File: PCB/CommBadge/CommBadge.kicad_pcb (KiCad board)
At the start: 2 copper layers, 49.3 x 39.8 mm, 46 parts, among them J1 Reset, J2 Battery, J3 TC2030-USB-NL-DS, J5 USB-C-Socket-H, Q1 CJ2301, SW2 SW_Push, U2 MAX98357A, U3 TP4054, U4 ME6211C33M5G-N, U5 L, U6 ESP32-S3-MINI-1, U7 R

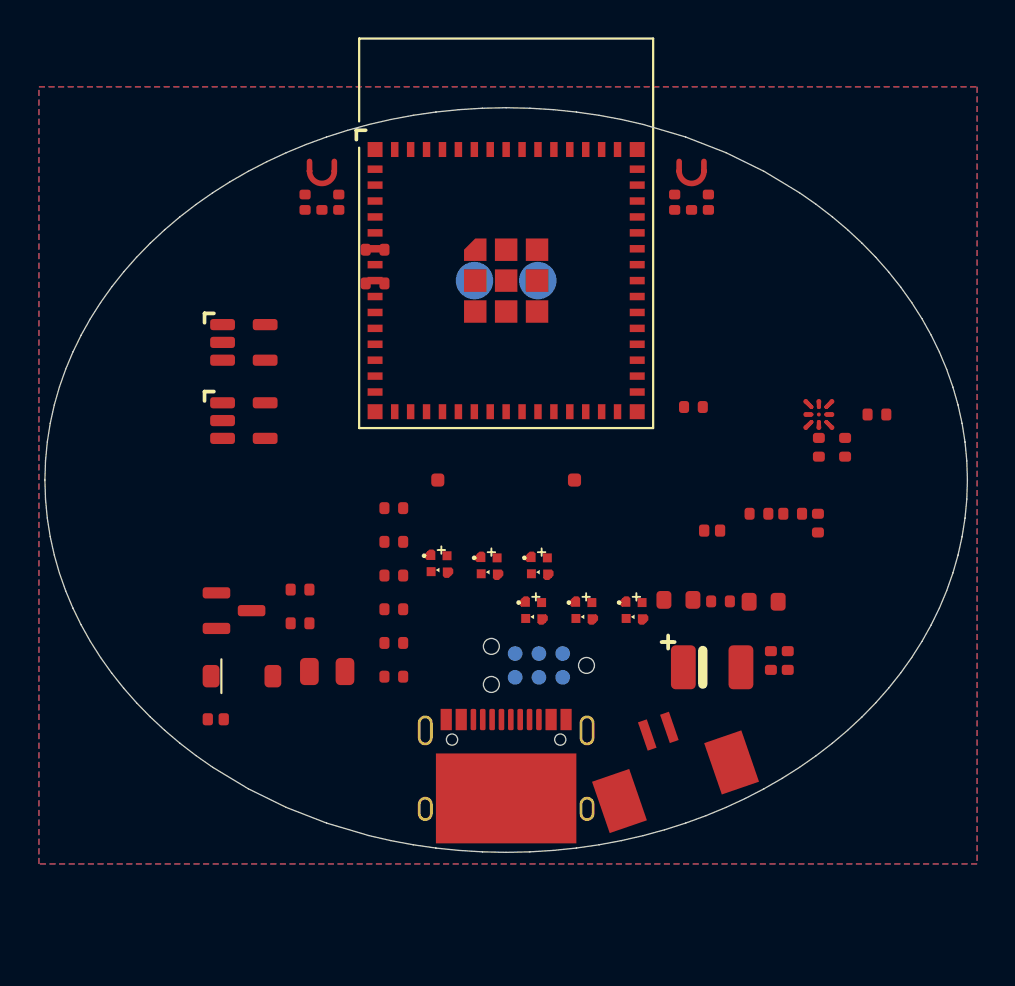
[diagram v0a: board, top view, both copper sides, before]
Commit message: Components
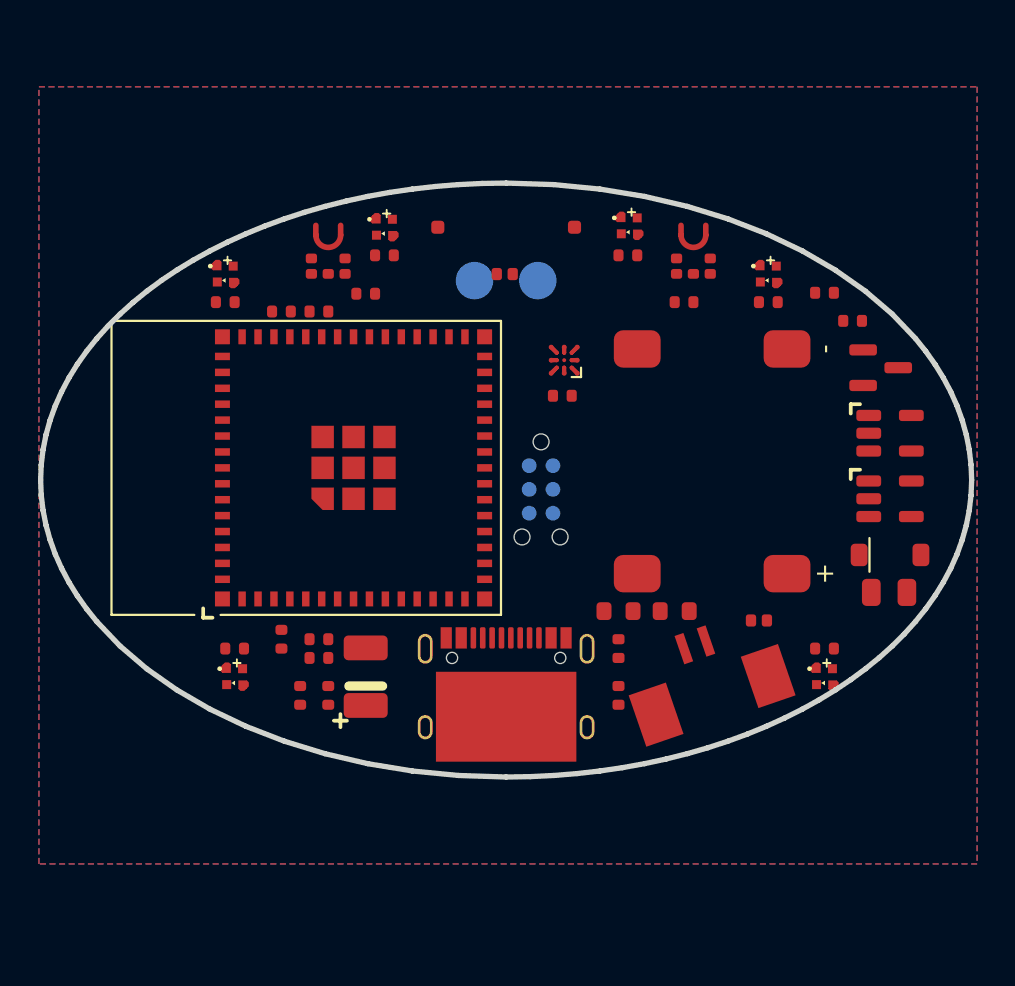
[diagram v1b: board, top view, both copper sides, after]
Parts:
- added LS1: Speaker, RevK:KLJ-Speaker, F.Cu at (111.0, 94.5)
- moved Q1 36.9 mm to (120.0, 89.5)
- moved D2 35.2 mm to (120.5, 99.5)
- moved U3 34.8 mm to (120.5, 93.0)
- moved U4 34.8 mm to (120.5, 96.5)
- moved R3 33.6 mm to (118.5, 87.0)
- moved R1 32.2 mm to (117.0, 85.5)
- moved C13 30.7 mm to (89.0, 107.0)
- moved C14 30.6 mm to (90.5, 107.0)
- moved C4 30.3 mm to (120.5, 101.5)
- moved D1 29.5 mm to (113.5, 103.0)
- moved C7 29.3 mm to (88.0, 104.0)
- moved D7 28.3 mm to (85.0, 84.5)
- moved C9 27.7 mm to (88.0, 86.5)
- moved R2 27.5 mm to (90.0, 86.5)
- moved C15 24.8 mm to (114.0, 86.0)
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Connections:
- C11 pad 1: Net-(D4-+) -> +3V3
- C11 pad 2: Net-(D4--) -> GND
- C12 pad 1: Net-(D4-+) -> +3V3
- C12 pad 2: Net-(D4--) -> GND
- C15 pad 1: Net-(D4-+) -> +3V3
- C15 pad 2: Net-(D4--) -> GND
- C16 pad 1: Net-(D4-+) -> +3V3
- C16 pad 2: Net-(D4--) -> GND
- C17 pad 1: Net-(D4-+) -> +3V3
- C17 pad 2: Net-(D4--) -> GND
- C18 pad 1: Net-(D4-+) -> +3V3
- C18 pad 2: Net-(D4--) -> GND
- C5 pad 1: DC -> VBUS
- D4 pad 2: Net-(D4-+) -> +3V3
- D4 pad 3: Net-(D4--) -> GND
- D5 pad 2: Net-(D4-+) -> +3V3
- D5 pad 3: Net-(D4--) -> GND
- D6 pad 2: Net-(D4-+) -> +3V3
- D6 pad 3: Net-(D4--) -> GND
- D7 pad 2: Net-(D4-+) -> +3V3
- D7 pad 3: Net-(D4--) -> GND
- D8 pad 2: Net-(D4-+) -> +3V3
- D8 pad 3: Net-(D4--) -> GND
- D9 pad 2: Net-(D4-+) -> +3V3
- D9 pad 3: Net-(D4--) -> GND
- J3 pad 1: DC -> VBUS
- J3 pad 2: DC -> VBUS
- J5 pad A4: DC -> VBUS
- J5 pad A9: DC -> VBUS
- J5 pad B4: DC -> VBUS
- J5 pad B9: DC -> VBUS
- U2 pad A3: unconnected-(U2-OUTP-PadA3) -> Net-(U2-OUTP)
- U2 pad B3: unconnected-(U2-OUTN-PadB3) -> Net-(U2-OUTN)
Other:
- board size 49.3 x 39.8 mm -> 49.7 x 31.7 mm

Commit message: Tweak
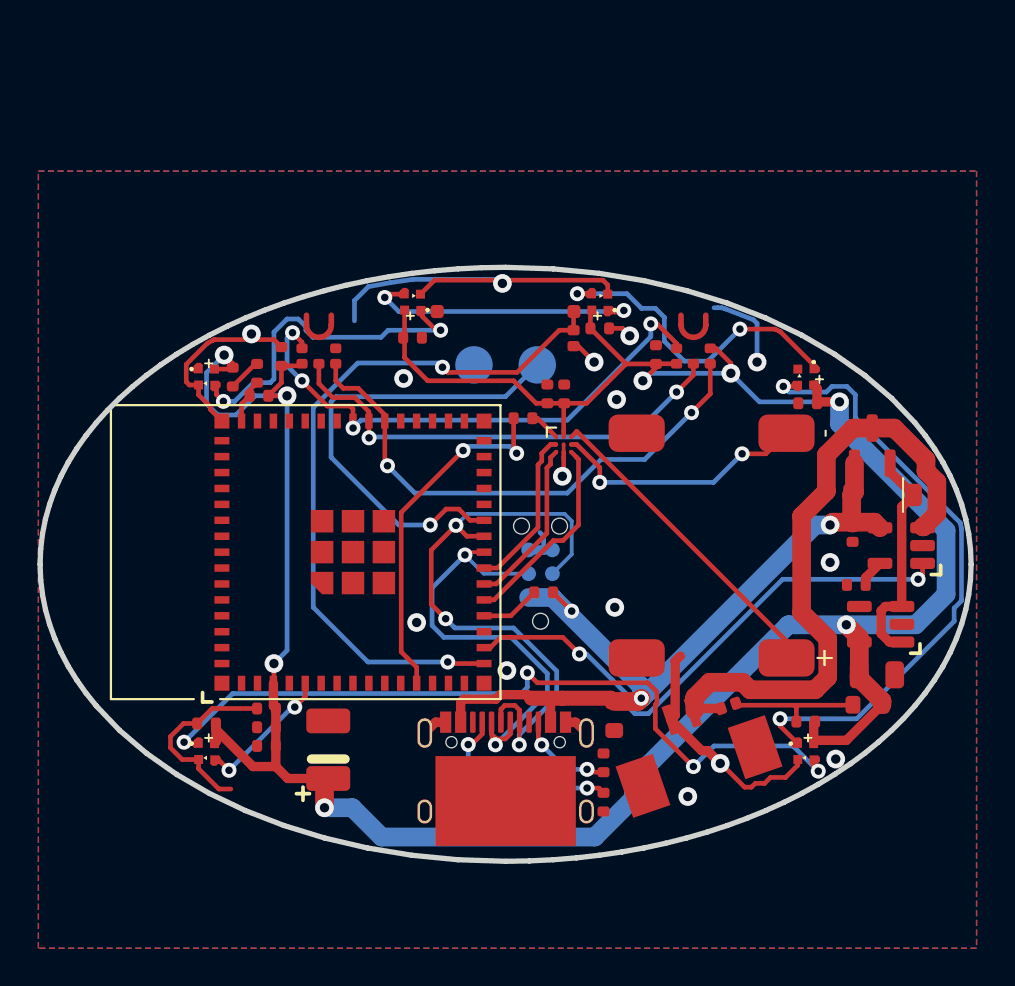
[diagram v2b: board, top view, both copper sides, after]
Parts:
- added R4: 10K, RevK:R_0402, F.Cu at (102.0, 101.5)
- moved C13 21.4 mm to (103.1, 90.9), turned to 90 degrees
- moved C14 19.9 mm to (102.2, 90.9), turned to 90 degrees
- moved R1 15.7 mm to (118.7, 101.1)
- moved C3 11.4 mm to (119.3, 107.5)
- moved R3 11.3 mm to (118.5, 98.3), turned to -90 degrees
- moved U4 6.72 mm to (120.0, 103.2), turned to 180 degrees
- moved R6 6.15 mm to (105.2, 110.6)
- moved U3 6.03 mm to (121.1, 99.0), turned to 180 degrees
- moved D5 5.85 mm to (116.0, 90.0), turned to -90 degrees
- moved C15 5.79 mm to (116.1, 91.4), turned to 180 degrees
- moved R5 5.76 mm to (105.2, 112.7), turned to -90 degrees
- moved C6 5.61 mm to (88.0, 88.9), turned to -90 degrees
- moved C5 5.60 mm to (105.8, 108.1), turned to -90 degrees
- moved D7 5.59 mm to (84.0, 90.0)
- moved R2 5.52 mm to (86.8, 91.0)
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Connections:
- D4 pad 4: RGB -> Net-(D4-I)
- D6 pad 4: Net-(D5-O) -> Net-(D6-I)
- D7 pad 1: Net-(D7-O) -> unconnected-(D7-O-Pad1)_1
- D8 pad 1: Net-(D8-O) -> Net-(D6-I)
- D8 pad 4: Net-(D7-O) -> Net-(D5-O)
- D9 pad 1: unconnected-(D9-O-Pad1) -> Net-(D4-I)
- D9 pad 4: Net-(D8-O) -> RGB
- U2 pad B2: unconnected-(U2-GAIN_SLOT-PadB2) -> GND
- U6 pad 10: RGB -> unconnected-(U6-GPIO6-Pad10)
- U6 pad 12: unconnected-(U6-GPIO8-Pad12) -> SKPPWR
- U6 pad 15: PUSH -> unconnected-(U6-GPIO11-Pad15)
- U6 pad 16: unconnected-(U6-GPIO12-Pad16) -> PUSH
- U6 pad 17: unconnected-(U6-GPIO13-Pad17) -> CHARGING
- U6 pad 19: unconnected-(U6-GPIO15-Pad19) -> Net-(U6-GPIO15)
- U6 pad 20: unconnected-(U6-GPIO16-Pad20) -> SKPWS
- U6 pad 21: unconnected-(U6-GPIO17-Pad21) -> SKPSCK
- U6 pad 22: unconnected-(U6-GPIO18-Pad22) -> SKPSD
- U6 pad 40: SKPPWR -> unconnected-(U6-GPIO44-Pad40)
- U6 pad 5: SKPWS -> RGB
- U6 pad 6: SKPSCK -> unconnected-(U6-GPIO2-Pad6)
- U6 pad 7: SKPSD -> unconnected-(U6-GPIO3-Pad7)
- U6 pad 8: RGB -> unconnected-(U6-GPIO4-Pad8)
- U6 pad 9: CHARGING -> unconnected-(U6-GPIO5-Pad9)
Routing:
- net +3V3: track 0.00 -> 148.1 mm, vias 0 -> 8
- net GND: track 0.00 -> 75.9 mm, vias 0 -> 15
- net VBUS: track 0.00 -> 43.0 mm, vias 0 -> 3
- net Net-(D4-I): track 0.00 -> 41.7 mm, vias 0 -> 4
- net PUSH: track 0.00 -> 38.1 mm, vias 0 -> 2
- net VBAT: track 0.00 -> 33.8 mm
- net D+: track 0.00 -> 33.0 mm, vias 0 -> 3
- net Net-(D4-O): track 0.00 -> 32.7 mm, vias 0 -> 2
- net CHARGING: track 0.00 -> 29.4 mm, vias 0 -> 2
- net MICSCK: track 0.00 -> 29.1 mm, vias 0 -> 4
- net MICWS: track 0.00 -> 28.7 mm, vias 0 -> 2
- net D-: track 0.00 -> 25.3 mm, vias 0 -> 2
- net MICSD: track 0.00 -> 25.1 mm, vias 0 -> 2
- net Net-(J1-Pin_2): track 0.00 -> 25.1 mm, vias 0 -> 1
- net SKPPWR: track 0.00 -> 19.2 mm, vias 0 -> 2
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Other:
- board text added: "1"
- board text added: "12"
- board text added: "13 15"
- board text added: "21"
- board text added: "40 41 42"
- board text added: "8 16 17 18"
- board text added: "A"
- board text added: "BTN"
- board text added: "Baking not required"
- board text added: "CHG VBUS"
- board text added: "LED"
- board text added: "MIC"
- board text added: "Made in China"
- board text added: "PWR WS SCK SD"
- board text added: "SPK"
- board text added: "WS SD SCK"
- board text added: "openmic.revk.uk"
- board text added: "®"
- board text removed: "Baking for D1 is not required"
